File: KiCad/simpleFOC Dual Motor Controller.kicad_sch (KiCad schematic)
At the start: 1 part, among them U101 STM32F103C8Tx

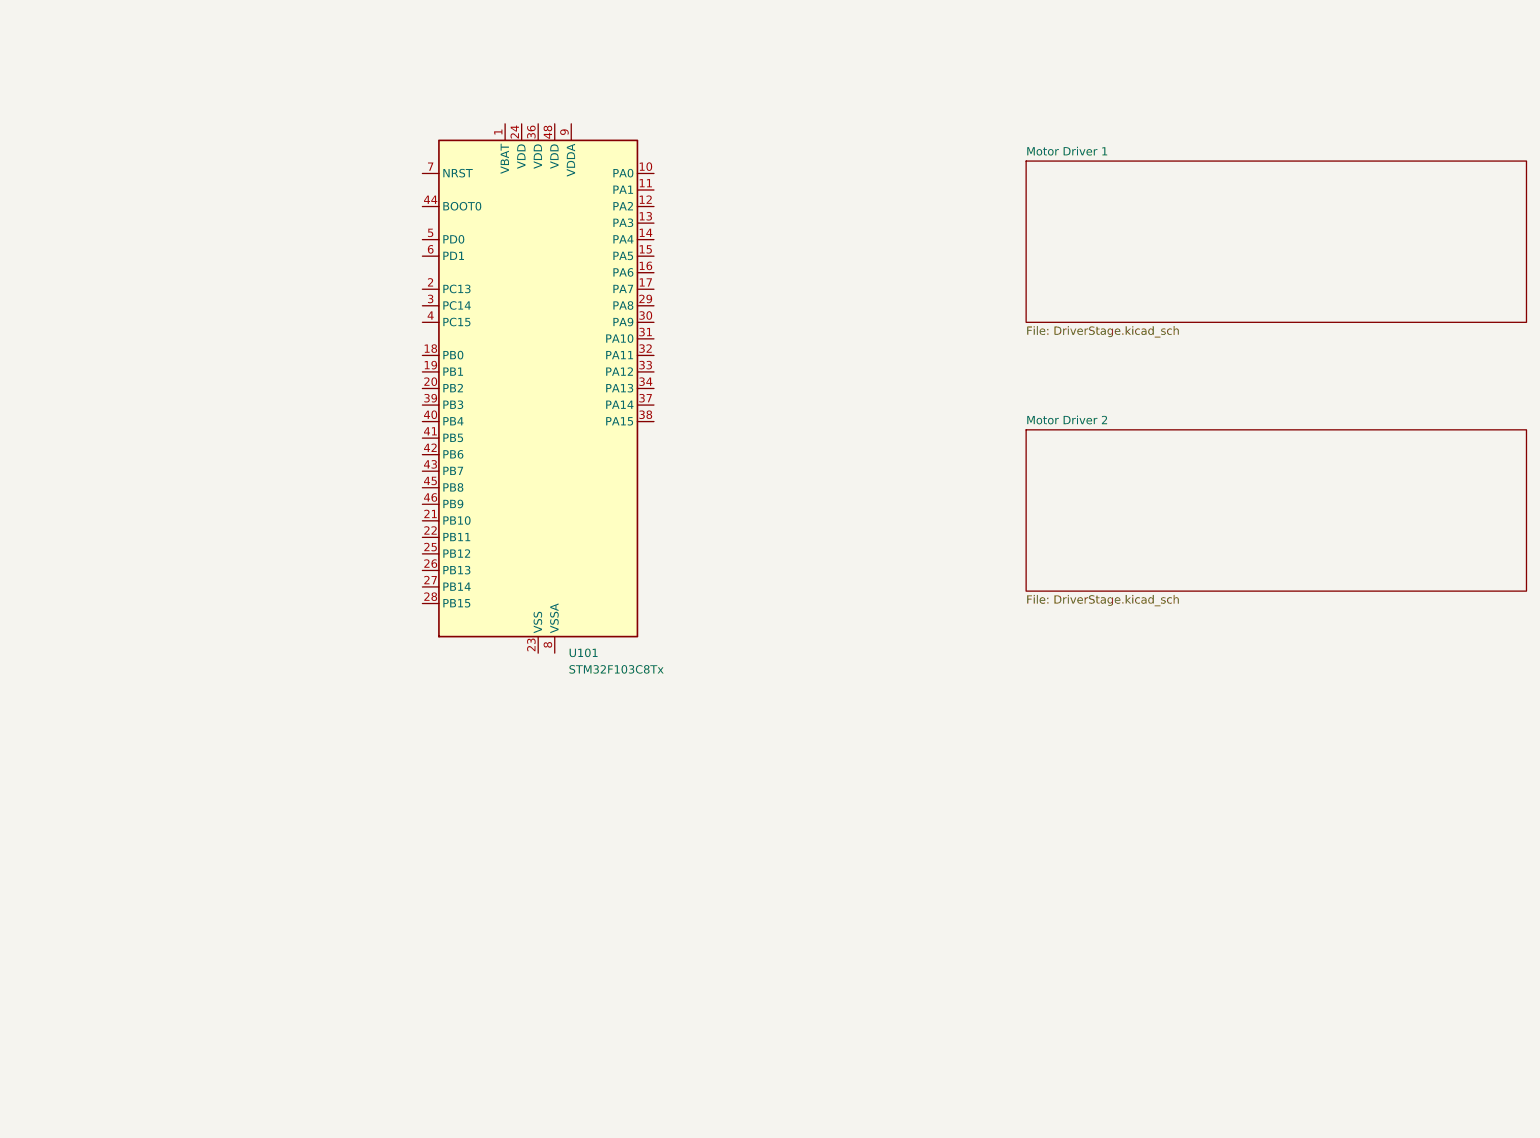
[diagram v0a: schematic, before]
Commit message: started adding supporting components
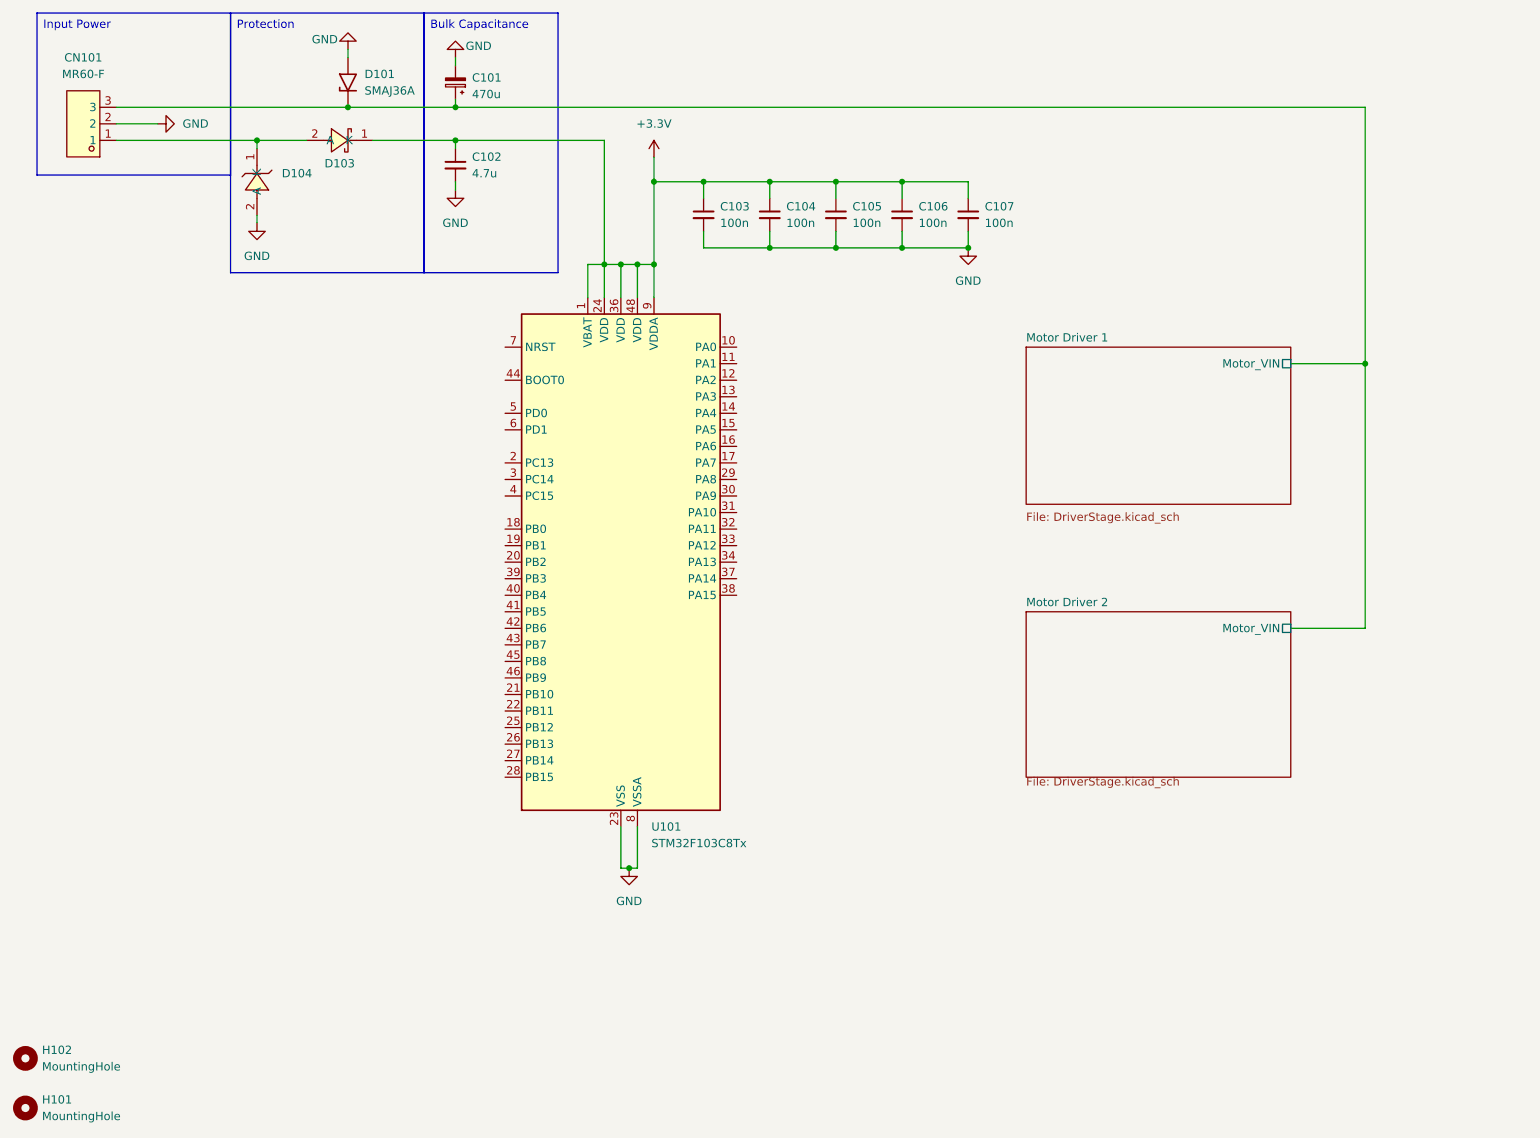
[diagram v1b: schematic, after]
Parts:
- added C101: 470u, symbol Device:C_Polarized_Small
- added C102: 4.7u, symbol Device:C_Small
- added C103, C104, C105, C106, C107: 100n, symbol Device:C_Small
- added CN101: MR60-F, easyeda2kicad:CONN-TH_3P-P5.50_MR60-F, symbol easyeda2kicad:MR60-F
- added D101: SMAJ36A, Diode_SMD:D_SMA, symbol Diode:SMAJ36A
- added D103: DSK26_C7502712, easyeda2kicad:SOD-123FL_L2.7-W1.8-LS3.8-RD, symbol easyeda2kicad:DSK26_C7502712
- added D104: SMF5.0A_C19077497, easyeda2kicad:SOD-123FL_L2.7-W1.8-LS3.8-RD, symbol easyeda2kicad:SMF5.0A_C19077497
- added H101, H102: MountingHole, MountingHole:MountingHole_4.3mm_M4, symbol Mechanical:MountingHole
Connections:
- net +3.3V: now reaches U101.1 (VBAT)
- net +3.3V: now also U101.24 (VDD), U101.36 (VDD), U101.48 (VDD), U101.9 (VDDA), C102.1, C103.1, C104.1, C105.1, C106.1, C107.1, D103.1 (K)
- net GND: now reaches U101.23 (VSS), U101.35 (VSS), U101.47 (VSS)
- net GND: now also U101.8 (VSSA), C101.2, C102.2, C103.2, C104.2, C105.2, C106.2, C107.2, CN101.2, D101.2 (A2), D104.2 (A)
- new net: CN101.1, D103.2 (A), D104.1 (K)
- new net Motor Driver 1/Motor_VIN: C101.1, CN101.3, D101.1 (A1)
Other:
- sheet Motor Driver 1 ports: added Motor_VIN; removed none
- sheet Motor Driver 2 ports: added Motor_VIN; removed none
- moved on the sheet: U101
